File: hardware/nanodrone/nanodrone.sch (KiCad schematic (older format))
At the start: 25 parts, among them J1 RTR0, J2 RTR1, J3 RTR2, J4 RTR3, Q1 SI2302, Q2 SI2302, Q3 SI2302, Q4 SI2302, U1 Feather

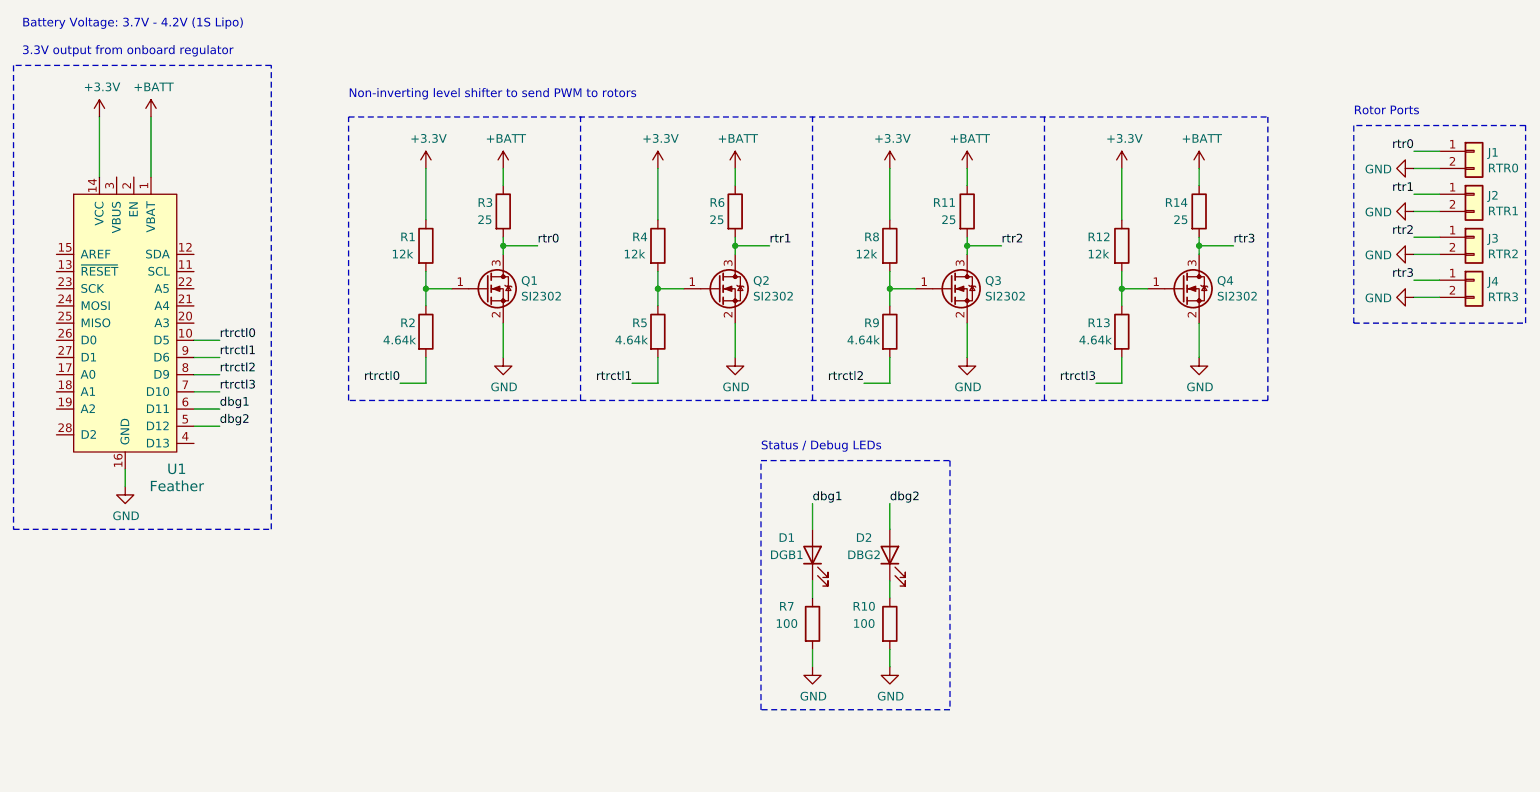
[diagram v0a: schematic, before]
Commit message: Rev D
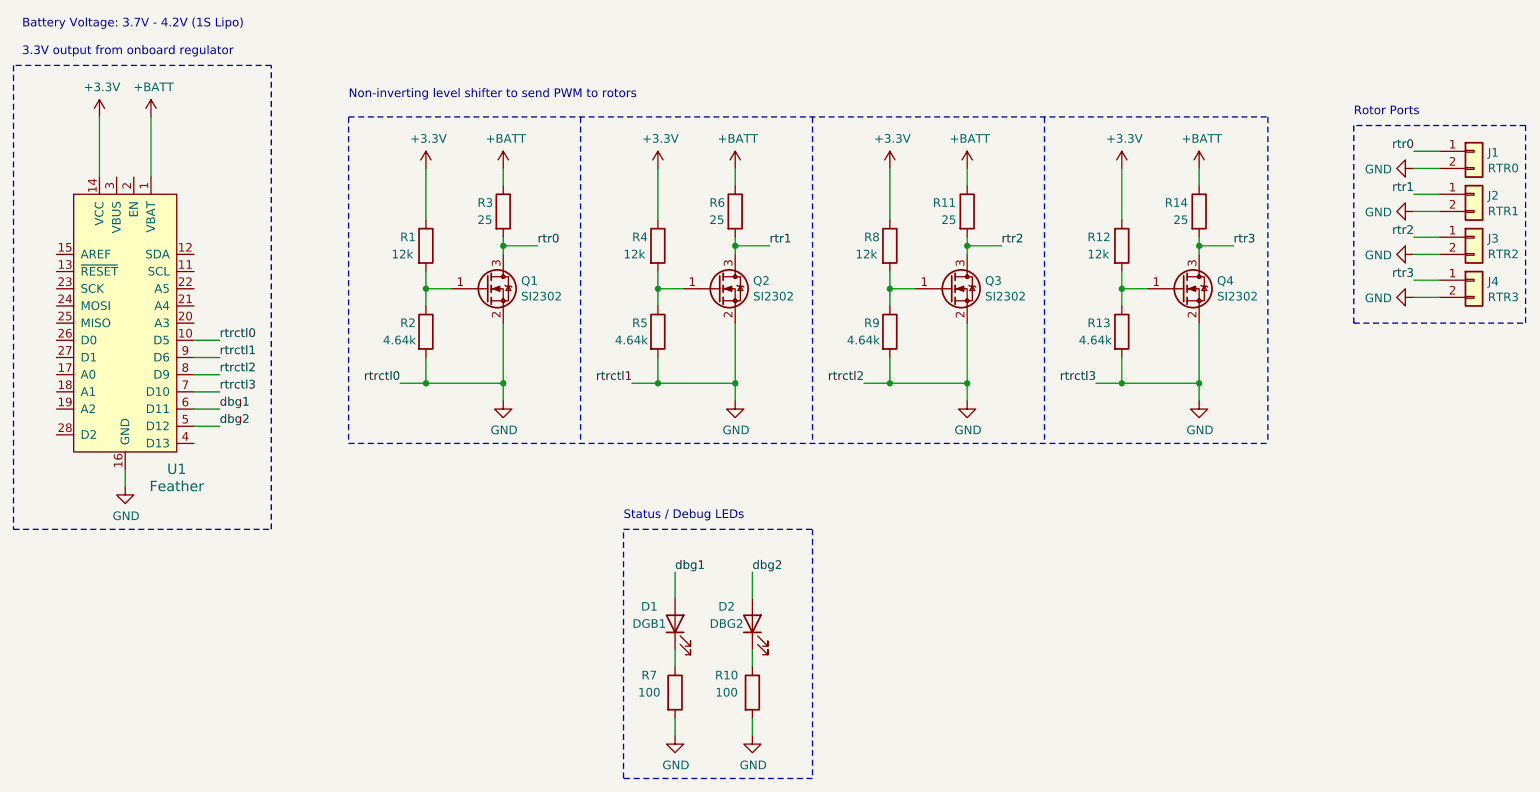
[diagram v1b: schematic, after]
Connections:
- net rtrctl0 is gone; now on net GND: R2.2, U1.10 (D5)
- net rtrctl1 is gone; now on net GND: R5.2, U1.9 (D6)
- net rtrctl2 is gone; now on net GND: R9.2, U1.8 (D9)
- net rtrctl3 is gone; now on net GND: R13.2, U1.7 (D10)
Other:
- moved on the sheet: D1, D2, R10, R7
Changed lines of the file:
@@
 L Device:LED D1
 U 1 1 613AA8FC
-P 6150 5300
-F 0 "D1" V 6250 5450 50  0000 C CNN
-F 1 "DGB1" V 6150 5450 50  0000 C CNN
-F 2 "LED_SMD:LED_0805_2012Metric" H 6150 5300 50  0001 C CNN
-F 3 "~" H 6150 5300 50  0001 C CNN
-F 4 "475-1410-2-ND" V 6150 5300 50  0001 C CNN "Digi-Key_PN"
-F 5 "C434432" V 6150 5300 50  0001 C CNN "LCSC Part Number"
-	1    6150 5300
+P 5350 5700
+F 0 "D1" V 5450 5850 50  0000 C CNN
+F 1 "DGB1" V 5350 5850 50  0000 C CNN
+F 2 "LED_SMD:LED_0805_2012Metric" H 5350 5700 50  0001 C CNN
+F 3 "~" H 5350 5700 50  0001 C CNN
+F 4 "475-1410-2-ND" V 5350 5700 50  0001 C CNN "Digi-Key_PN"
+F 5 "C434432" V 5350 5700 50  0001 C CNN "LCSC Part Number"
+	1    5350 5700
 	0    -1   -1   0
 $EndComp
@@
 L Device:LED D2
 U 1 1 613AAEC3
-P 6600 5300
-F 0 "D2" V 6700 5450 50  0000 C CNN
-F 1 "DBG2" V 6600 5450 50  0000 C CNN
-F 2 "LED_SMD:LED_0805_2012Metric_Pad1.15x1.40mm_HandSolder" H 6600 5300 50  0001 C CNN
-F 3 "~" H 6600 5300 50  0001 C CNN
-F 4 "475-1410-2-ND" V 6600 5300 50  0001 C CNN "Digi-Key_PN"
-F 5 "C434432" V 6600 5300 50  0001 C CNN "LSCS Part Number"
-	1    6600 5300
+P 5800 5700
+F 0 "D2" V 5900 5850 50  0000 C CNN
+F 1 "DBG2" V 5800 5850 50  0000 C CNN
+F 2 "LED_SMD:LED_0805_2012Metric_Pad1.15x1.40mm_HandSolder" H 5800 5700 50  0001 C CNN
+F 3 "~" H 5800 5700 50  0001 C CNN
+F 4 "475-1410-2-ND" V 5800 5700 50  0001 C CNN "Digi-Key_PN"
+F 5 "C434432" V 5800 5700 50  0001 C CNN "LSCS Part Number"
+	1    5800 5700
 	0    -1   -1   0
 $EndComp
@@
 L Device:R R7
 U 1 1 613AC424
-P 6150 5700
-F 0 "R7" H 6000 5800 50  0000 C CNN
-F 1 "100" H 6000 5700 50  0000 C CNN
-F 2 "Resistor_SMD:R_0805_2012Metric_Pad1.15x1.40mm_HandSolder" V 6080 5700 50  0001 C CNN
-F 3 "~" H 6150 5700 50  0001 C CNN
-F 4 "P100ATR-ND" H 6150 5700 50  0001 C CNN "Digi-Key_PN"
-F 5 "C17408" H 6150 5700 50  0001 C CNN "LCSC Part Number"
-	1    6150 5700
+P 5350 6100
+F 0 "R7" H 5200 6200 50  0000 C CNN
+F 1 "100" H 5200 6100 50  0000 C CNN
+F 2 "Resistor_SMD:R_0805_2012Metric_Pad1.15x1.40mm_HandSolder" V 5280 6100 50  0001 C CNN
+F 3 "~" H 5350 6100 50  0001 C CNN
+F 4 "P100ATR-ND" H 5350 6100 50  0001 C CNN "Digi-Key_PN"
+F 5 "C17408" H 5350 6100 50  0001 C CNN "LCSC Part Number"
+	1    5350 6100
 	1    0    0    -1
 $EndComp
@@
 L Device:R R10
 U 1 1 613ACDB5
-P 6600 5700
-F 0 "R10" H 6450 5800 50  0000 C CNN
-F 1 "100" H 6450 5700 50  0000 C CNN
-F 2 "Resistor_SMD:R_0805_2012Metric_Pad1.15x1.40mm_HandSolder" V 6530 5700 50  0001 C CNN
-F 3 "~" H 6600 5700 50  0001 C CNN
-F 4 "P100ATR-ND" H 6600 5700 50  0001 C CNN "Digi-Key_PN"
-F 5 "C17408" H 6600 5700 50  0001 C CNN "LCSC Part Number"
-	1    6600 5700
-	1    0    0    -1
-$EndComp
-Wire Wire Line
-	6150 5550 6150 5450
-Wire Wire Line
-	6600 5550 6600 5450
+P 5800 6100
+F 0 "R10" H 5650 6200 50  0000 C CNN
+F 1 "100" H 5650 6100 50  0000 C CNN
+F 2 "Resistor_SMD:R_0805_2012Metric_Pad1.15x1.40mm_HandSolder" V 5730 6100 50  0001 C CNN
+F 3 "~" H 5800 6100 50  0001 C CNN
+F 4 "P100ATR-ND" H 5800 6100 50  0001 C CNN "Digi-Key_PN"
+F 5 "C17408" H 5800 6100 50  0001 C CNN "LCSC Part Number"
+	1    5800 6100
+	1    0    0    -1
+$EndComp
+Wire Wire Line
+	5350 5950 5350 5850
+Wire Wire Line
+	5800 5950 5800 5850
 $Comp
 L power:GND #PWR01
 U 1 1 613B4116
-P 6150 5950
-F 0 "#PWR01" H 6150 5700 50  0001 C CNN
-F 1 "GND" H 6155 5777 50  0000 C CNN
-F 2 "" H 6150 5950 50  0001 C CNN
-F 3 "" H 6150 5950 50  0001 C CNN
-	1    6150 5950
+P 5350 6350
+F 0 "#PWR01" H 5350 6100 50  0001 C CNN
+F 1 "GND" H 5355 6177 50  0000 C CNN
+F 2 "" H 5350 6350 50  0001 C CNN
+F 3 "" H 5350 6350 50  0001 C CNN
+	1    5350 6350
 	1    0    0    -1
 $EndComp
@@
 L power:GND #PWR02
 U 1 1 613B4CBB
-P 6600 5950
-F 0 "#PWR02" H 6600 5700 50  0001 C CNN
-F 1 "GND" H 6605 5777 50  0000 C CNN
-F 2 "" H 6600 5950 50  0001 C CNN
-F 3 "" H 6600 5950 50  0001 C CNN
-	1    6600 5950
-	1    0    0    -1
-$EndComp
-Wire Wire Line
-	6150 5950 6150 5850
-Wire Wire Line
-	6600 5950 6600 5850
-Wire Wire Line
-	6150 5150 6150 5000
+P 5800 6350
+F 0 "#PWR02" H 5800 6100 50  0001 C CNN
+F 1 "GND" H 5805 6177 50  0000 C CNN
+F 2 "" H 5800 6350 50  0001 C CNN
+F 3 "" H 5800 6350 50  0001 C CNN
+	1    5800 6350
+	1    0    0    -1
+$EndComp
+Wire Wire Line
+	5350 6350 5350 6250
+Wire Wire Line
+	5800 6350 5800 6250
+Wire Wire Line
+	5350 5550 5350 5400
 Text Notes 9300 2750 0    50   ~ 0
 Rotor Ports
-Text Notes 5850 4700 0    50   ~ 0
+Text Notes 5050 5100 0    50   ~ 0
 Status / Debug LEDs
 Wire Wire Line
-	6600 5150 6600 5000
+	5800 5550 5800 5400
 Wire Wire Line
 	2550 4050 2700 4050
@@
 	3000 2450 1500 2450
 Wire Notes Line
-	5850 4750 6950 4750
-Wire Notes Line
-	6950 4750 6950 6200
-Wire Notes Line
-	6950 6200 5850 6200
-Wire Notes Line
-	5850 6200 5850 4750
+	5050 5150 6150 5150
+Wire Notes Line
+	6150 5150 6150 6600
+Wire Notes Line
+	6150 6600 5050 6600
+Wire Notes Line
+	5050 6600 5050 5150
 Wire Notes Line
 	9300 2800 9300 3950
@@
 Text Label 2700 4550 0    50   ~ 0
 dbg2
-Text Label 6150 5000 0    50   ~ 0
+Text Label 5350 5400 0    50   ~ 0
 dbg1
-Text Label 6600 5000 0    50   ~ 0
+Text Label 5800 5400 0    50   ~ 0
 dbg2
 $Comp
@@
 L power:GND #PWR03
 U 1 1 6196904D
-P 4350 4150
-F 0 "#PWR03" H 4350 3900 50  0001 C CNN
-F 1 "GND" H 4355 3977 50  0000 C CNN
-F 2 "" H 4350 4150 50  0001 C CNN
-F 3 "" H 4350 4150 50  0001 C CNN
-	1    4350 4150
-	1    0    0    -1
-$EndComp
-Wire Wire Line
-	4350 4150 4350 3950
+P 4350 4400
+F 0 "#PWR03" H 4350 4150 50  0001 C CNN
+F 1 "GND" H 4355 4227 50  0000 C CNN
+F 2 "" H 4350 4400 50  0001 C CNN
+F 3 "" H 4350 4400 50  0001 C CNN
+	1    4350 4400
+	1    0    0    -1
+$EndComp
 Wire Wire Line
 	3750 4300 3900 4300
@@
 L power:GND #PWR06
 U 1 1 619BFE47
-P 5700 4150
-F 0 "#PWR06" H 5700 3900 50  0001 C CNN
-F 1 "GND" H 5705 3977 50  0000 C CNN
-F 2 "" H 5700 4150 50  0001 C CNN
-F 3 "" H 5700 4150 50  0001 C CNN
-	1    5700 4150
-	1    0    0    -1
-$EndComp
-Wire Wire Line
-	5700 4150 5700 3950
+P 5700 4400
+F 0 "#PWR06" H 5700 4150 50  0001 C CNN
+F 1 "GND" H 5705 4227 50  0000 C CNN
+F 2 "" H 5700 4400 50  0001 C CNN
+F 3 "" H 5700 4400 50  0001 C CNN
+	1    5700 4400
+	1    0    0    -1
+$EndComp
 Wire Wire Line
 	5100 4300 5250 4300
@@
 L power:GND #PWR09
 U 1 1 619C620B
-P 7050 4150
-F 0 "#PWR09" H 7050 3900 50  0001 C CNN
-F 1 "GND" H 7055 3977 50  0000 C CNN
-F 2 "" H 7050 4150 50  0001 C CNN
-F 3 "" H 7050 4150 50  0001 C CNN
-	1    7050 4150
-	1    0    0    -1
-$EndComp
-Wire Wire Line
-	7050 4150 7050 3950
+P 7050 4400
+F 0 "#PWR09" H 7050 4150 50  0001 C CNN
+F 1 "GND" H 7055 4227 50  0000 C CNN
+F 2 "" H 7050 4400 50  0001 C CNN
+F 3 "" H 7050 4400 50  0001 C CNN
+	1    7050 4400
+	1    0    0    -1
+$EndComp
 Wire Wire Line
 	6450 4300 6600 4300
@@
 L power:GND #PWR012
 U 1 1 619CC4B9
-P 8400 4150
-F 0 "#PWR012" H 8400 3900 50  0001 C CNN
-F 1 "GND" H 8405 3977 50  0000 C CNN
-F 2 "" H 8400 4150 50  0001 C CNN
-F 3 "" H 8400 4150 50  0001 C CNN
-	1    8400 4150
-	1    0    0    -1
-$EndComp
-Wire Wire Line
-	8400 4150 8400 3950
+P 8400 4400
+F 0 "#PWR012" H 8400 4150 50  0001 C CNN
+F 1 "GND" H 8405 4227 50  0000 C CNN
+F 2 "" H 8400 4400 50  0001 C CNN
+F 3 "" H 8400 4400 50  0001 C CNN
+	1    8400 4400
+	1    0    0    -1
+$EndComp
 Wire Wire Line
 	7800 4300 7950 4300
@@
 	7950 3350 7950 3050
 Wire Notes Line
-	3450 4400 3450 2750
-Wire Notes Line
 	3450 2750 8800 2750
-Wire Notes Line
-	8800 2750 8800 4400
-Wire Notes Line
-	8800 4400 3450 4400
-Wire Notes Line
-	4800 4400 4800 2750
-Wire Notes Line
-	6150 4400 6150 2750
-Wire Notes Line
-	7500 4400 7500 2750
 $Comp
 L Transistor_FET:2N7002E Q1
@@
 	1    0    0    -1
 $EndComp
+Wire Wire Line
+	4350 4400 4350 4300
+Connection ~ 4350 4300
+Wire Wire Line
+	4350 4300 4350 3950
+Wire Wire Line
+	3900 4300 4350 4300
+Connection ~ 3900 4300
+Wire Wire Line
+	5700 4400 5700 4300
+Wire Wire Line
+	7050 4400 7050 4300
+Wire Wire Line
+	8400 4400 8400 4300
+Wire Wire Line
+	7950 4300 8400 4300
+Connection ~ 7950 4300
+Connection ~ 8400 4300
+Wire Wire Line
+	8400 4300 8400 3950
+Wire Wire Line
+	6600 4300 7050 4300
+Connection ~ 6600 4300
+Connection ~ 7050 4300
+Wire Wire Line
+	7050 4300 7050 3950
+Wire Wire Line
+	5250 4300 5700 4300
+Connection ~ 5250 4300
+Connection ~ 5700 4300
+Wire Wire Line
+	5700 4300 5700 3950
+Wire Notes Line
+	3450 4650 8800 4650
+Wire Notes Line
+	3450 2750 3450 4650
+Wire Notes Line
+	8800 2750 8800 4650
+Wire Notes Line
+	4800 2750 4800 4650
+Wire Notes Line
+	6150 2750 6150 4650
+Wire Notes Line
+	7500 2750 7500 4650
 $EndSCHEMATC
